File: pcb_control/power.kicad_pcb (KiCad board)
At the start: 2 copper layers, 24.1 x 31.8 mm, 12 parts, among them J1 PWR OFF, J2 VOUT, J3 GND, J4 VIN, J5 PWR BTN, Q1 Q_PMOS_GDS, Q2 Q_NMOS_GDS

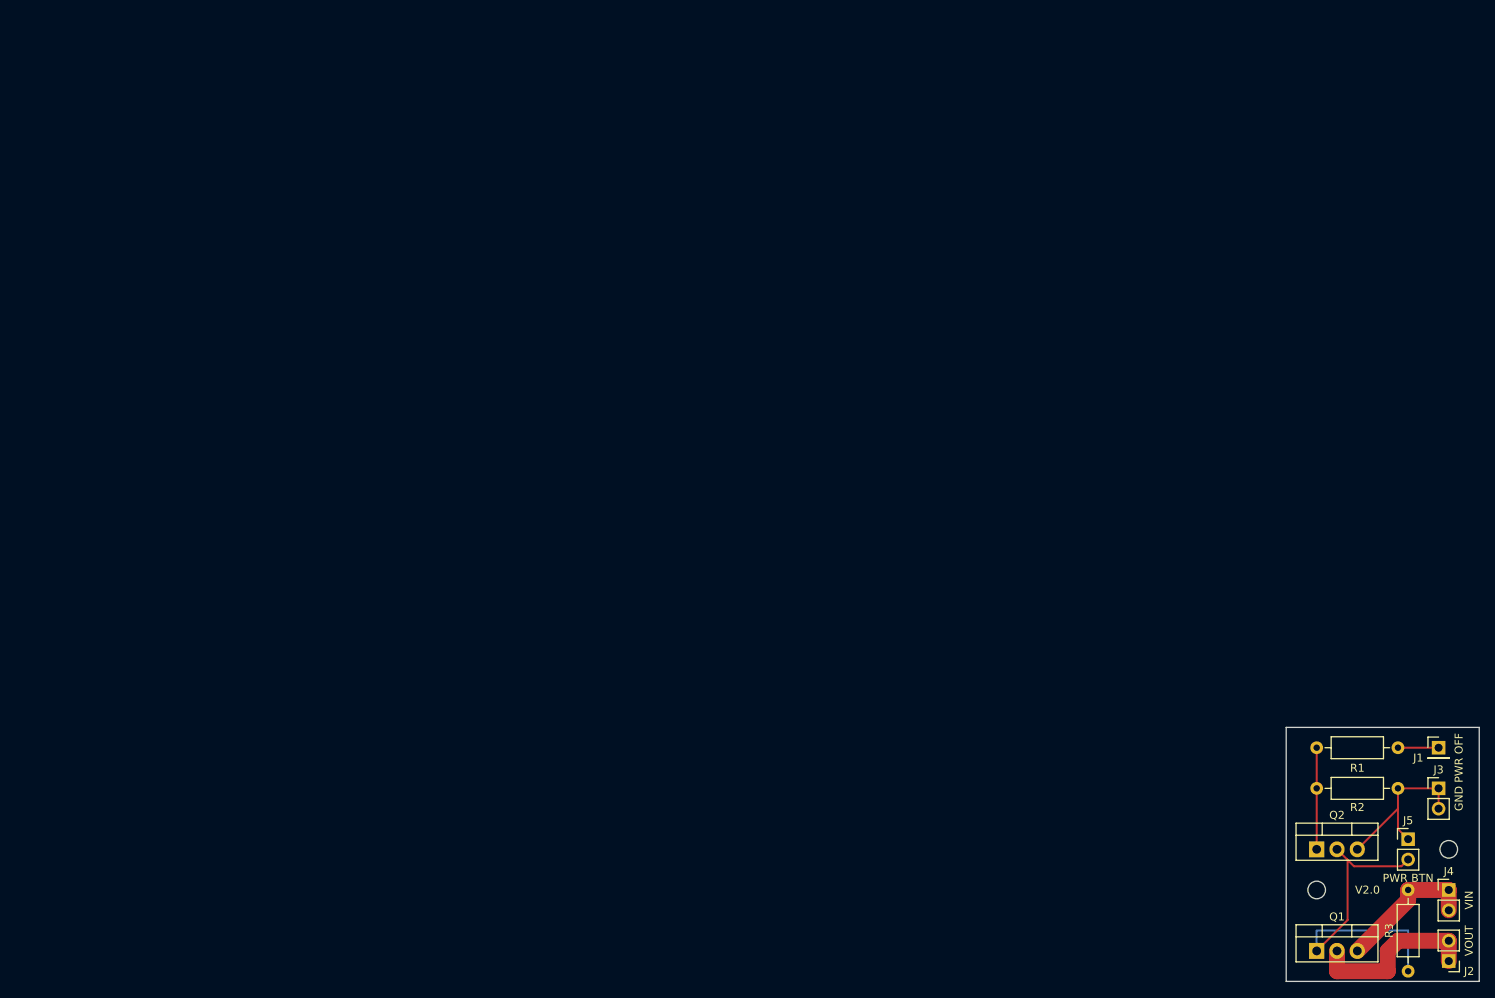
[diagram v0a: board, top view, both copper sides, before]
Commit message: wip
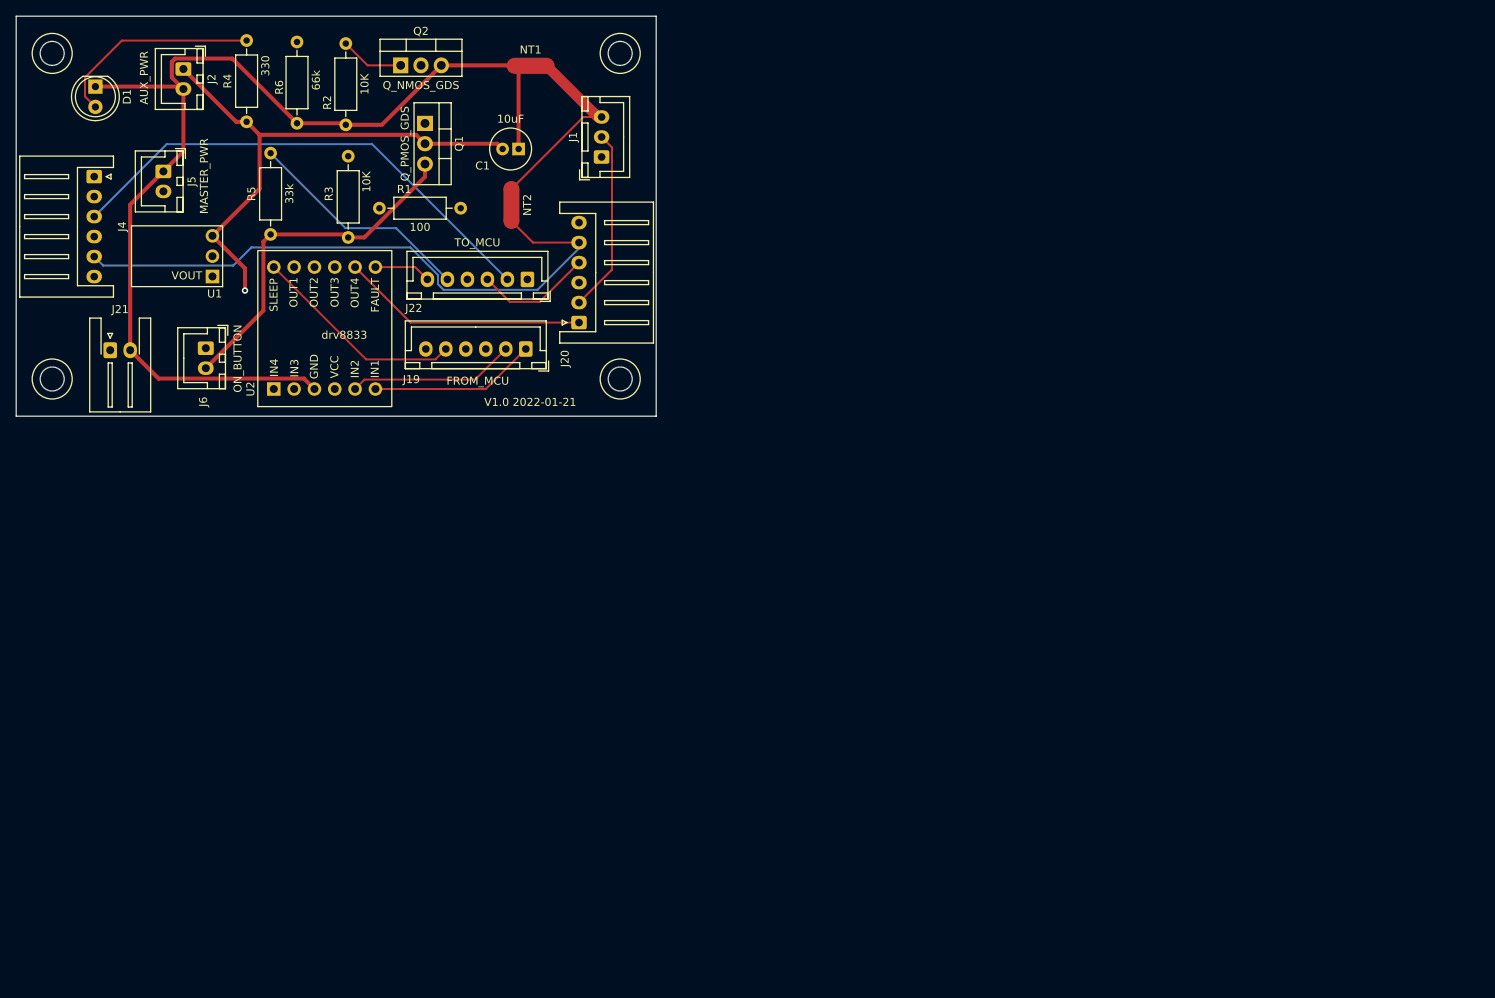
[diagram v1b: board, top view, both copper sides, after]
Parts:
- removed J3: GND, Connector_PinHeader_2.54mm:PinHeader_1x02_P2.54mm_Vertical
- removed REF** (x2): MountingHole_2.2mm_M2, MountingHole:MountingHole_2.2mm_M2
- added C1: 10uF, Capacitor_THT:C_Radial_D5.0mm_H11.0mm_P2.00mm, F.Cu at (62.8, 16.6)
- added D1: LED, LED_THT:LED_D5.0mm, F.Cu at (9.90, 8.80)
- added J19: FROM_MCU, Connector_JST:JST_XH_B6B-XH-A_1x06_P2.50mm_Vertical, F.Cu at (63.7, 41.6)
- added J20: M_RGT, Connector_JST:JST_XH_S6B-XH-A_1x06_P2.50mm_Horizontal, F.Cu at (70.3, 38.3)
- added J21: BAT, Connector_JST:JST_XH_S2B-XH-A-1_1x02_P2.50mm_Horizontal, F.Cu at (11.8, 41.8)
- added J22: TO_MCU, Connector_JST:JST_XH_B6B-XH-A_1x06_P2.50mm_Vertical, F.Cu at (63.9, 32.9)
- added J6: MASTER_PWR_SW, Connector_JST:JST_XH_B2B-XH-A_1x02_P2.50mm_Vertical, F.Cu at (23.7, 41.5)
- added NT1: NetTi, NetTie:NetTie-2_SMD_Pad2.0mm, F.Cu at (64.3, 6.20)
- added NT2: NetTie_2, NetTie:NetTie-2_SMD_Pad2.0mm, F.Cu at (61.9, 23.6)
- added R4: 330, Resistor_THT:R_Axial_DIN0207_L6.3mm_D2.5mm_P10.16mm_Horizontal, F.Cu at (28.8, 13.2)
- added R5: 33k, Resistor_THT:R_Axial_DIN0207_L6.3mm_D2.5mm_P10.16mm_Horizontal, F.Cu at (31.8, 27.3)
- added R6: 66k, Resistor_THT:R_Axial_DIN0207_L6.3mm_D2.5mm_P10.16mm_Horizontal, F.Cu at (35.1, 3.22)
- added U1: S9V11F5, tobi:pololu_5v_updown, F.Cu at (25.8, 33.8)
- added U2: DRV8833, tobi:drv8833, F.Cu at (32.2, 46.6)
- J1: value PWR OFF -> MCU_PWR; footprint Connector_PinHeader_2.54mm:PinHeader_1x01_P2.54mm_Vertical -> Connector_JST:JST_XH_B3B-XH-A_1x03_P2.50mm_Vertical
- J2: value VOUT -> AUX_VOUT; footprint Connector_PinHeader_2.54mm:PinHeader_1x02_P2.54mm_Vertical -> Connector_JST:JST_XH_B2B-XH-A_1x02_P2.50mm_Vertical
- J4: value VIN -> M_LFT; footprint Connector_PinHeader_2.54mm:PinHeader_1x02_P2.54mm_Vertical -> Connector_JST:JST_XH_S6B-XH-A_1x06_P2.50mm_Horizontal
- J5: footprint Connector_PinHeader_2.54mm:PinHeader_1x02_P2.54mm_Vertical -> Connector_JST:JST_XH_B2B-XH-A_1x02_P2.50mm_Vertical
- moved J2 193.5 mm to (20.9, 6.60), turned to -90 degrees
- moved J4 191.4 mm to (9.75, 20.1), turned to -90 degrees
- moved J5 176.6 mm to (18.4, 19.4), turned to -90 degrees
- moved R3 167.1 mm to (41.5, 17.5), turned to -90 degrees
- moved R2 155.5 mm to (41.2, 13.6), turned to 90 degrees
- moved Q1 152.1 mm to (51.1, 13.4), turned to -90 degrees
- moved Q2 150.7 mm to (48.1, 6.14)
- moved R1 135.2 mm to (45.4, 24.0)
- moved J1 128.1 mm to (73.2, 17.6), turned to 90 degrees
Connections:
- J2 pad 1: VCC -> /XYZ
- J2 pad 2: VCC -> /GND1
- J4 pad 1: +BATT -> Net-(J4-Pad1)
- J4 pad 2: +BATT -> Net-(J1-Pad2)
- J5 pad 1: GND -> /GND1
- Q1 pad 2: VCC -> /XYZ
- Q1 pad 3: +BATT -> /BAT2
- Q2 pad 3: GND -> /GND1
- R2 pad 1: GND -> /GND1
- R3 pad 2: +BATT -> /BAT2
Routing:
- net /GND1: track 0.00 -> 135.3 mm
- net Net-(J1-Pad2): track 0.00 -> 89.0 mm
- net /XYZ: track 0.00 -> 84.6 mm, vias 0 -> 1
- net Net-(J1-Pad3): track 0.00 -> 80.4 mm
- net Net-(J20-Pad5): track 0.00 -> 77.3 mm
- net Net-(J22-Pad2): track 0.00 -> 62.4 mm
- net Net-(J22-Pad1): track 0.00 -> 60.6 mm
- net /BAT2: track 0.00 -> 44.3 mm
- net Net-(J22-Pad5): track 0.00 -> 43.9 mm
- net Net-(J4-Pad1): track 0.00 -> 32.9 mm
- net Net-(J20-Pad6): track 0.00 -> 32.8 mm
- net Net-(J20-Pad1): track 0.00 -> 30.9 mm
- net Net-(J19-Pad3): track 0.00 -> 27.0 mm
- net Net-(J19-Pad5): track 0.00 -> 26.8 mm
- net Net-(J4-Pad6): track 0.00 -> 26.5 mm
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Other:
- board size 24.1 x 31.8 mm -> 80 x 50 mm
- copper layers 2 -> 4
- net class Default removed
- board text added: "AUX_PWR"
- board text added: "MASTER_PWR"
- board text added: "ON_BUTTON"
- board text added: "V1.0 2022-01-21"
- board text removed: "V2.0"
